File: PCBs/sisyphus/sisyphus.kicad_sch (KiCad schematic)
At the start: 65 parts, among them J1 USB_C_Receptacle_USB2.0_14P, J2 AUX USB, J3 Conn_01x02, J4 Speaker, J5 SWD, J6 RGB_CONN, J7 Keyboard, J8 Light sensor, J9 Battery, U1 NCP1117-3.3_SOT223, U2 USBLC6-2P6, U3 W25Q128JVS, U4 MAX98357A, U5 RP2040, U7 BQ25619, Y1 ABM8-272-T3

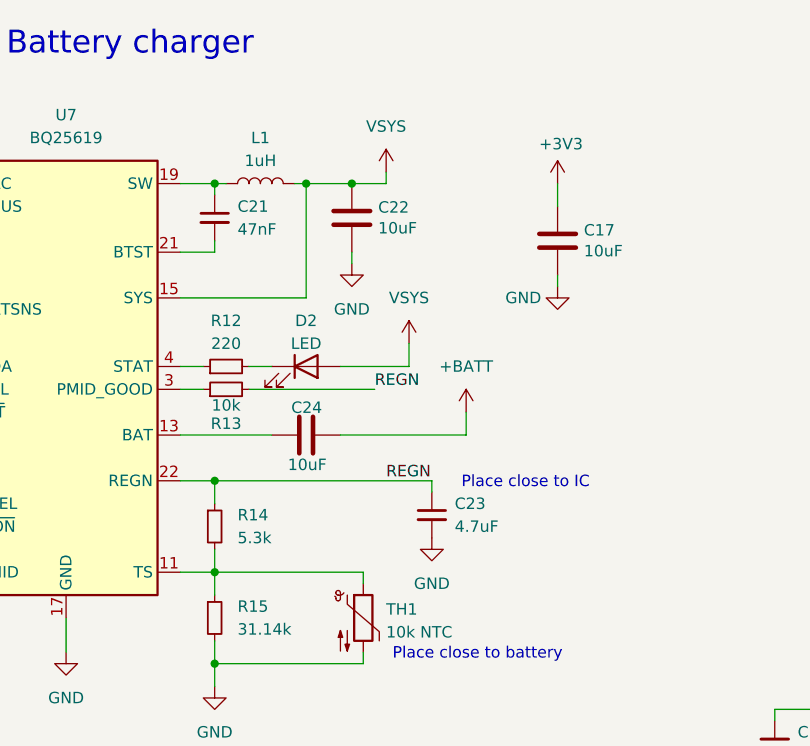
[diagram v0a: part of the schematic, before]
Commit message: Update main PCB
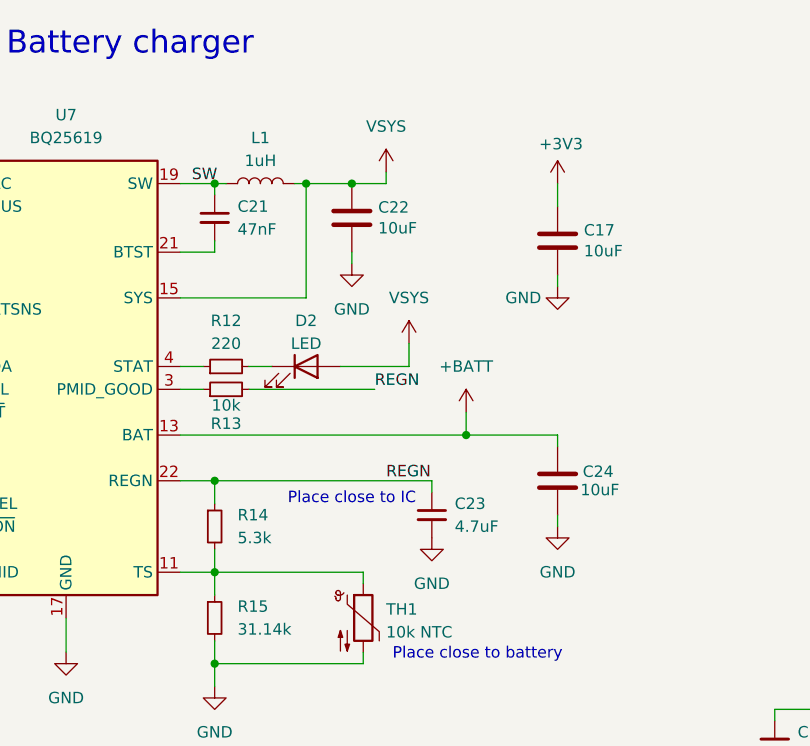
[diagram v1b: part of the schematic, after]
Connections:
- net +BATT: now also C24.1, U7.13 (BAT), U7.14 (BAT); no longer C24.2
- net GND: now also C24.2
- net SW: now reaches C21.1, L1.1, U7.19 (SW), U7.20 (SW)
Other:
- moved on the sheet: C24
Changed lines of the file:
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@@
 	(text "Place close to IC"
 		(exclude_from_sim no)
-		(at 294.894 72.644 0)
+		(at 275.59 74.422 0)
 		(effects
 			(font
@@
 	)
 	(junction
+		(at 288.29 67.31)
+		(diameter 0)
+		(color 0 0 0 0)
+	)
+	(junction
 		(at 180.34 36.83)
 		(diameter 0)
@@
 	(wire
 		(pts
+			(xy 288.29 67.31) (xy 298.45 67.31)
+		)
+		(stroke
+			(width 0)
+			(type default)
+		)
+	)
+	(wire
+		(pts
 			(xy 203.2 139.7) (xy 205.74 139.7)
 		)
@@
 	(wire
 		(pts
-			(xy 274.32 67.31) (xy 288.29 67.31)
-		)
-		(stroke
-			(width 0)
-			(type default)
-		)
-	)
-	(wire
-		(pts
 			(xy 170.18 36.83) (xy 180.34 36.83)
 		)
@@
 	(wire
 		(pts
-			(xy 256.54 67.31) (xy 266.7 67.31)
+			(xy 256.54 67.31) (xy 288.29 67.31)
 		)
 		(stroke
@@
 	(wire
 		(pts
+			(xy 298.45 67.31) (xy 298.45 68.58)
+		)
+		(stroke
+			(width 0)
+			(type default)
+		)
+	)
+	(wire
+		(pts
 			(xy 100.33 243.84) (xy 113.03 243.84)
 		)
@@
 	(wire
 		(pts
+			(xy 298.45 76.2) (xy 298.45 77.47)
+		)
+		(stroke
+			(width 0)
+			(type default)
+		)
+	)
+	(wire
+		(pts
 			(xy 237.49 198.12) (xy 247.65 198.12)
 		)
@@
 		)
 	)
+	(label "SW"
+		(at 257.81 39.37 0)
+		(effects
+			(font
+				(size 1.27 1.27)
+			)
+			(justify left bottom)
+		)
+	)
 	(label "DN"
 		(at 96.52 63.5 180)
@@
 	)
 	(symbol
+		(lib_name "GND_8")
+		(lib_id "power:GND")
+		(at 298.45 77.47 0)
+		(unit 1)
+		(exclude_from_sim no)
+		(in_bom yes)
+		(on_board yes)
+		(dnp no)
+		(fields_autoplaced yes)
+		(property "Reference" "#PWR055"
+			(at 298.45 83.82 0)
+			(effects
+				(font
+					(size 1.27 1.27)
+				)
+				(hide yes)
+			)
+		)
+		(property "Value" "GND"
+			(at 298.45 82.55 0)
+			(effects
+				(font
+					(size 1.27 1.27)
+				)
+			)
+		)
+		(property "Footprint" ""
+			(at 298.45 77.47 0)
+			(effects
+				(font
+					(size 1.27 1.27)
+				)
+				(hide yes)
+			)
+		)
+		(property "Datasheet" ""
+			(at 298.45 77.47 0)
+			(effects
+				(font
+					(size 1.27 1.27)
+				)
+				(hide yes)
+			)
+		)
+		(property "Description" "Power symbol creates a global label with name \"GND\" , ground"
+			(at 298.45 77.47 0)
+			(effects
+				(font
+					(size 1.27 1.27)
+				)
+				(hide yes)
+			)
+		)
+		(pin "1"
+		)
+		(instances
+			(project "sisyphus"
+				(path "/8c0b3d8b-46d3-4173-ab1e-a61765f77d61"
+					(reference "#PWR055")
+					(unit 1)
+				)
+			)
+		)
+	)
+	(symbol
 		(lib_id "Device:R_Small")
 		(at 250.19 198.12 90)
@@
 	(symbol
 		(lib_id "Device:C")
-		(at 270.51 67.31 90)
+		(at 298.45 72.39 0)
 		(unit 1)
 		(exclude_from_sim no)
@@
 		(dnp no)
 		(property "Reference" "C24"
-			(at 272.288 64.262 90)
+			(at 301.244 71.374 0)
 			(effects
 				(font
@@
 		)
 		(property "Value" "10uF"
-			(at 272.796 70.612 90)
+			(at 300.99 73.406 0)
 			(effects
 				(font
@@
 		)
 		(property "Footprint" "Capacitor_SMD:C_0805_2012Metric"
-			(at 274.32 66.3448 0)
+			(at 299.4152 76.2 0)
 			(effects
 				(font
@@
 		)
 		(property "Datasheet" "~"
-			(at 270.51 67.31 0)
+			(at 298.45 72.39 0)
 			(effects
 				(font
@@
 		)
 		(property "Description" ""
-			(at 270.51 67.31 0)
+			(at 298.45 72.39 0)
 			(effects
 				(font
